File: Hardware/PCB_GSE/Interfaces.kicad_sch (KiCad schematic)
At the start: 34 parts, among them J1 Conn_01x02, J2 BM03B-GHS-TBT, J3 GT17HN-4DP-2H(D)(56), J5 Screw_Terminal_01x04, U2 ISOW1044, U3 SI5442DU-T1-GE3, U6 SI5442DU-T1-GE3, U7 SI5442DU-T1-GE3, X1 Conn_02x07_Odd_Even

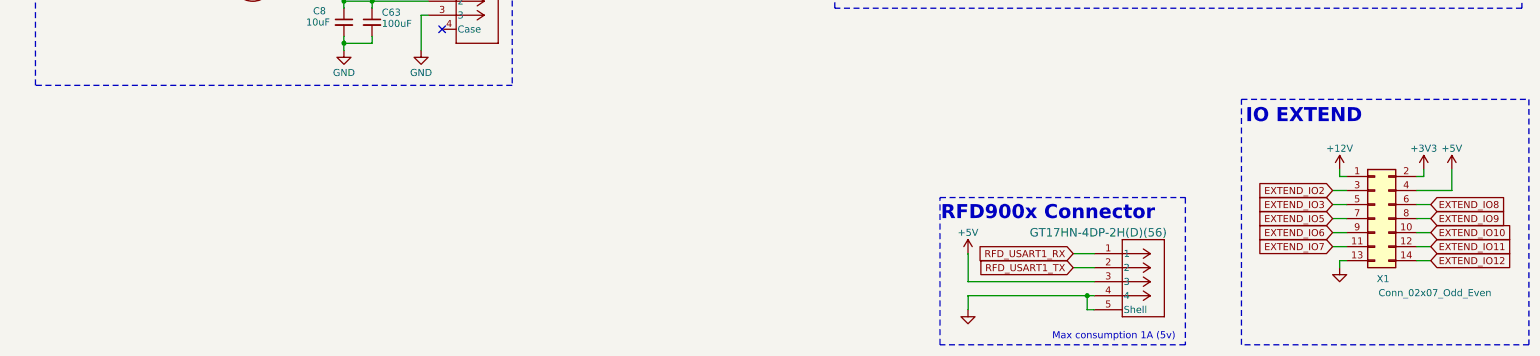
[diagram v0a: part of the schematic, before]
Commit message: feature : Done v1 and send to fab
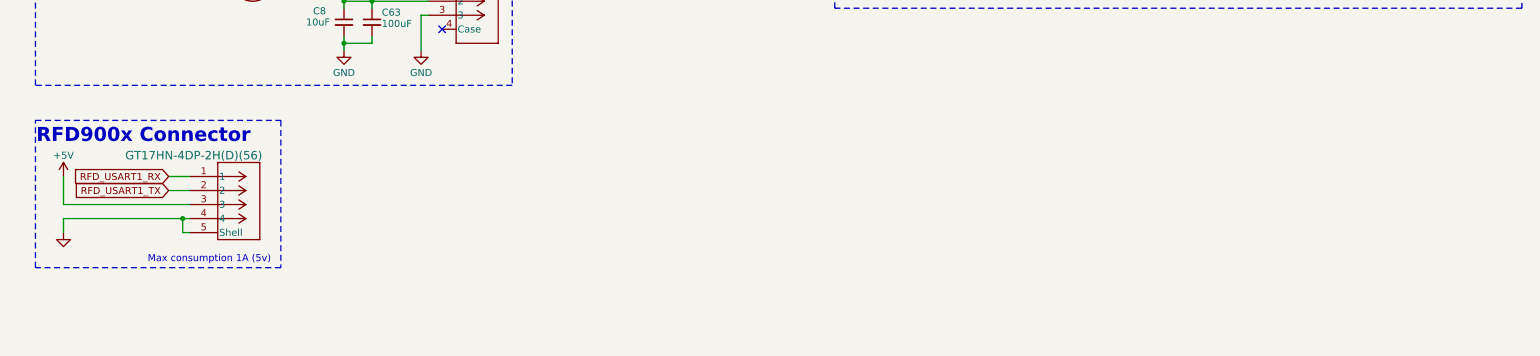
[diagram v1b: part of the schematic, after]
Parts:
- removed X1: Conn_02x07_Odd_Even, Connector_PinHeader_2.54mm:PinHeader_2x07_P2.54mm_Vertical, symbol Connector_Generic:Conn_02x07_Odd_Even
- C3, C9: DigiKey_Part_Number 399-C0603C105K4RACTUCT-ND -> 1276-1029-1-ND; Manufacturer_Part_Number C0603C105K4RACTU -> CL21B105KBFNNNE
- J2: value BM03B-GHS-TBT -> SM03B-GHS-TB; DigiKey_Part_Number (none) -> 455-SM03B-GHS-TBCT-ND; Manufacturer_Part_Number (none) -> SM03B-GHS-TB
- R11, R14, R3: DigiKey_Part_Number 311-10.0KHRCT-ND -> 541-10.0KCCT-ND; Manufacturer_Part_Number RC0603FR-0710KL -> CRCW080510K0FKEA
- R5: DigiKey_Part_Number P1.5KDBCT-ND -> 311-1.50KCRCT-ND; Manufacturer_Part_Number ERA-3AEB152V -> RC0805FR-071K5L
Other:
- note removed: "IO EXTEND"
